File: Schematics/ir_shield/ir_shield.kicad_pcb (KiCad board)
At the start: 4 copper layers, 68.6 x 53.3 mm, 51 parts, among them Q1 Q_Photo_NPN, Q2 Q_Photo_NPN, Q3 Q_Photo_NPN, Q4 Q_Photo_NPN, Q5 Q_NMOS, U1 LM6132

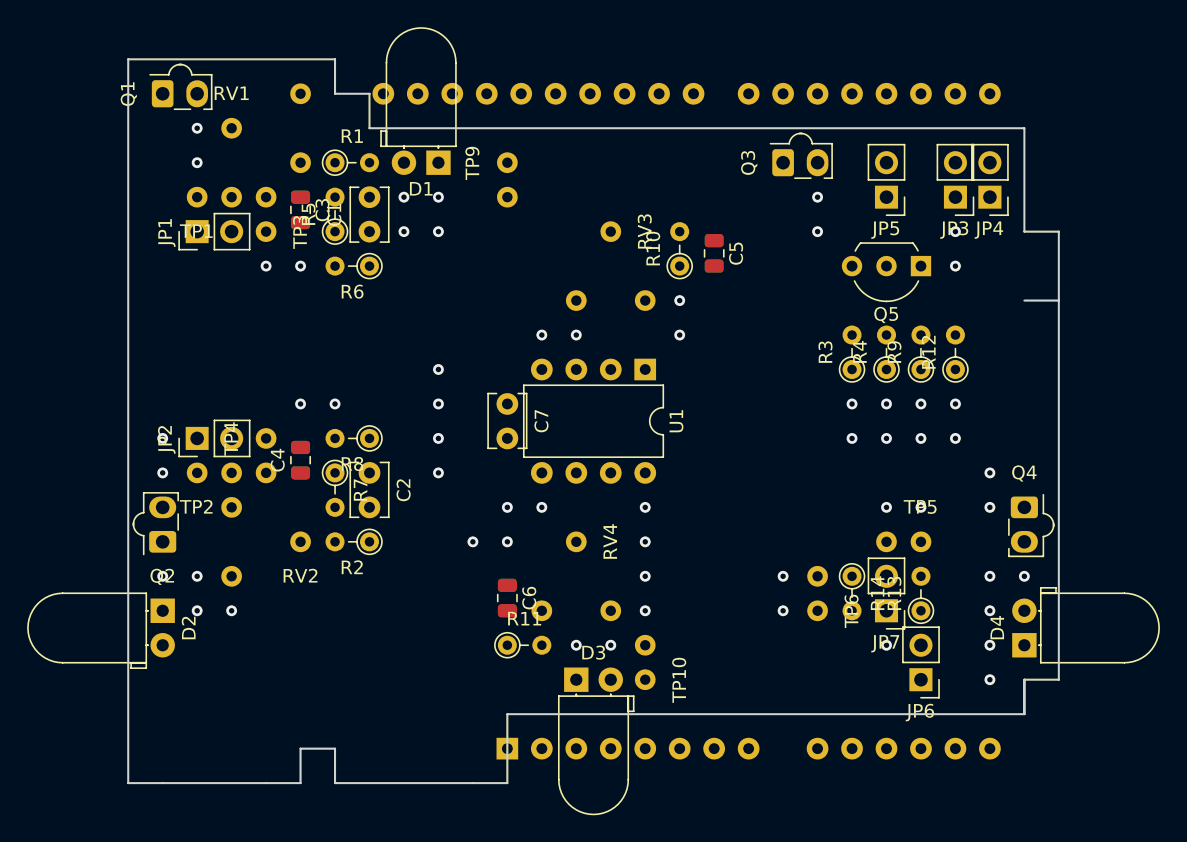
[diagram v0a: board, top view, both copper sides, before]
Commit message: added some changes
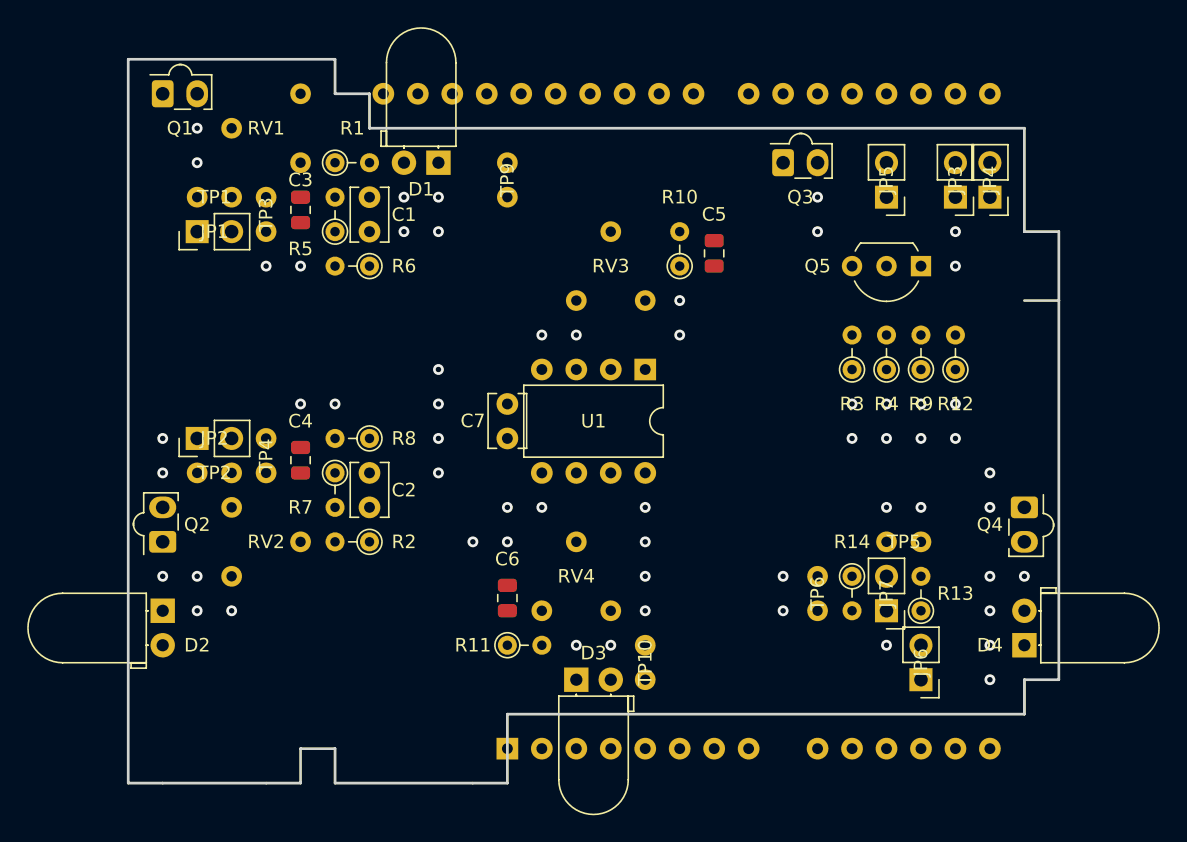
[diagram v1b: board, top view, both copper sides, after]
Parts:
- R10, R11: value 100R -> 2k
- RV3, RV4: value 100k -> 20k
